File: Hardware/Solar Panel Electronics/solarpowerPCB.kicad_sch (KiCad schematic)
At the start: 45 parts, among them J3 Conn_01x02_Male, J4 Conn_01x06_Male, J5 Conn_01x02_Male, Q1 MMDT2222A, U1 SN65HVD230, U2 ESP32-PICO-D4

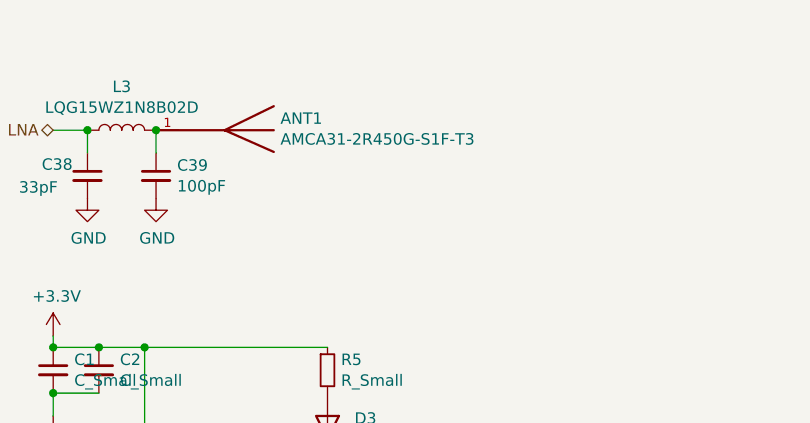
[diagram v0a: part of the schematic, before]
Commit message: Preliminary Layout done. (46x77mm)
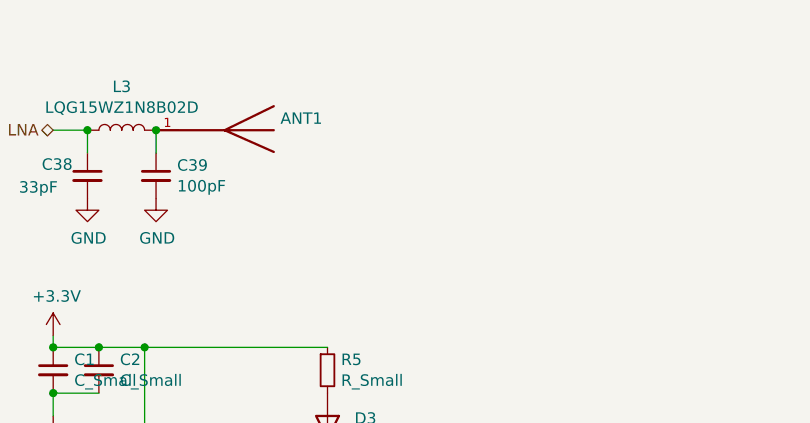
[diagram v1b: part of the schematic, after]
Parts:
- ANT1: value AMCA31-2R450G-S1F-T3 -> (none); footprint iclr:ANT_AMCA31-2R450G-S1F-T3 -> (none)
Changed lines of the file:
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@@
       (effects (font (size 1.27 1.27)) (justify left))
     )
-    (property "Value" "AMCA31-2R450G-S1F-T3" (id 1) (at 154.7876 27.686 90)
+    (property "Value" "" (id 1) (at 154.7876 27.686 90)
       (effects (font (size 1.27 1.27)) (justify left))
     )
-    (property "Footprint" "iclr:ANT_AMCA31-2R450G-S1F-T3" (id 2) (at 146.05 26.67 0)
+    (property "Footprint" "" (id 2) (at 146.05 26.67 0)
       (effects (font (size 1.27 1.27)) (justify left bottom) hide)
     )

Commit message: Layed out parts a bit more
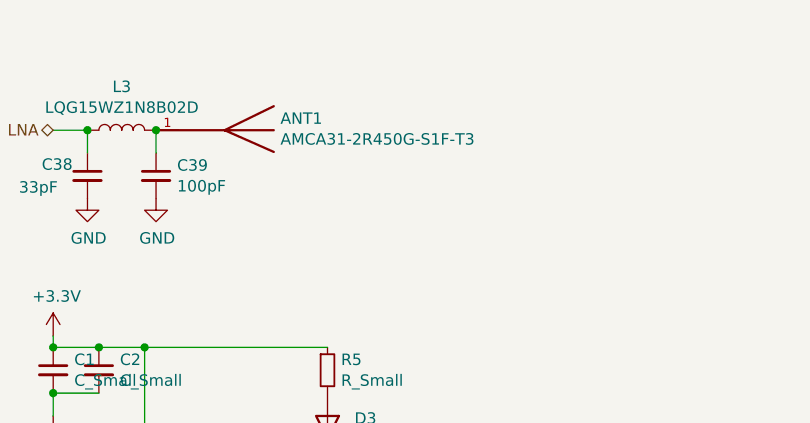
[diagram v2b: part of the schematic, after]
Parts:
- ANT1: value (none) -> AMCA31-2R450G-S1F-T3; footprint (none) -> iclr:ANT_AMCA31-2R450G-S1F-T3
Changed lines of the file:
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@@
       (effects (font (size 1.27 1.27)) (justify left))
     )
-    (property "Value" "" (id 1) (at 154.7876 27.686 90)
+    (property "Value" "AMCA31-2R450G-S1F-T3" (id 1) (at 154.7876 27.686 90)
       (effects (font (size 1.27 1.27)) (justify left))
     )
-    (property "Footprint" "" (id 2) (at 146.05 26.67 0)
+    (property "Footprint" "iclr:ANT_AMCA31-2R450G-S1F-T3" (id 2) (at 146.05 26.67 0)
       (effects (font (size 1.27 1.27)) (justify left bottom) hide)
     )
